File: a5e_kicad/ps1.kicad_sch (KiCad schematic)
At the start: 63 parts, among them U16 AP61202Z6, U18 AP61202Z6, U19 AP61202Z6, U8 AP61202Z6

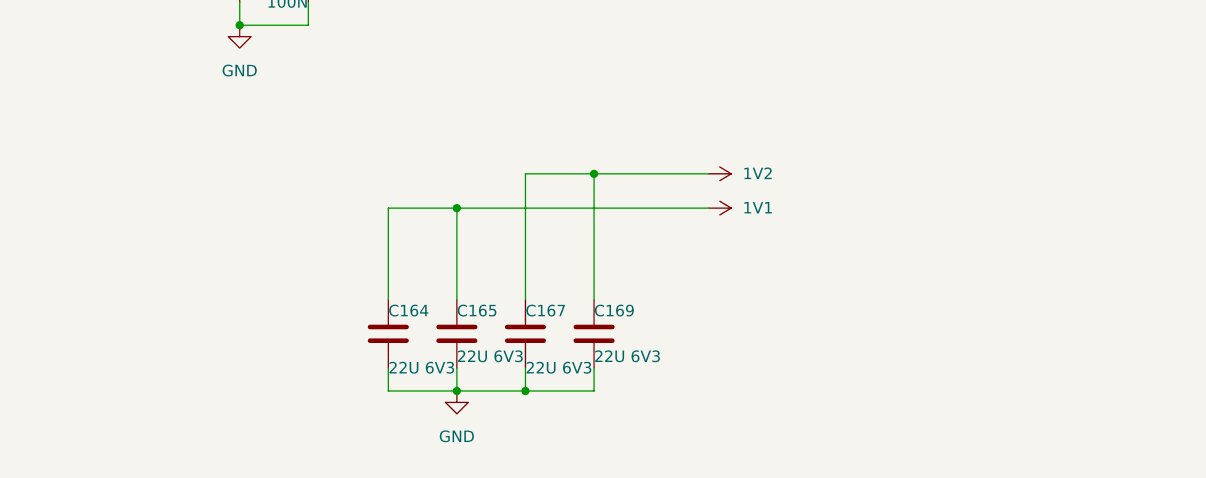
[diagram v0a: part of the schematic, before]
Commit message: more fiddling with aux power supplies
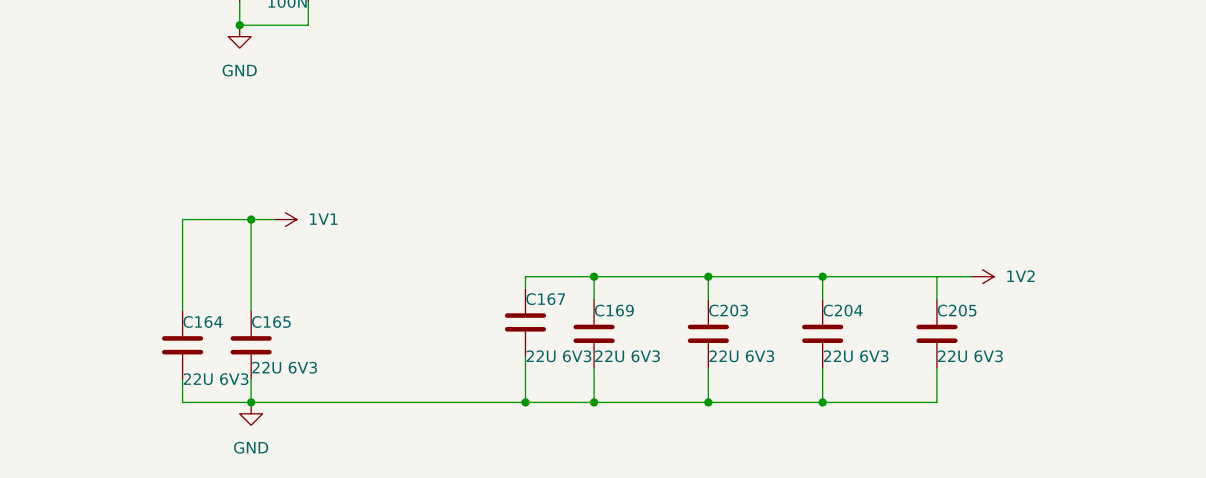
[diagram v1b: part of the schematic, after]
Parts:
- added C203, C204, C205: 22U 6V3, Capacitor_SMD:C_0402_1005Metric, symbol Device:C
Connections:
- net 1V2: now also C203.1, C204.1
- net GND: now also C203.2, C204.2, C205.2
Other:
- moved on the sheet: C164, C165, C167
